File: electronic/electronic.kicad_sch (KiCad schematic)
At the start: 63 parts, among them J1 POWER SUPLY, J10 MOT_W_ENCODER03, J11 Conn_01x02, J12 Conn_01x02, J13 Conn_01x02, J14 DRVO01, J15 DRVO01, J16 Screw_Terminal_01x03, J17 Conn_01x04, J18 Conn_01x02, J19 Conn_01x02, J2 MOT_W_ENCODER01, J20 Conn_01x02, J21 DRVO01, J22 Screw_Terminal_01x03, J23 DRVO01, J24 Conn_01x04, J25 Conn_01x05, J26 Conn_01x04, J27 Conn_01x04, J28 Conn_01x05, J3 M01, J4 ENC01, J5 M02, J6 ENC02, J7 MOT_W_ENCODER02, J8 M03, J9 ENC03, U1 ESP32-S3-DevKitC, U2 L298N, U3 LM78M05_TO252, U4 L298N, U5 LM78M05_TO252

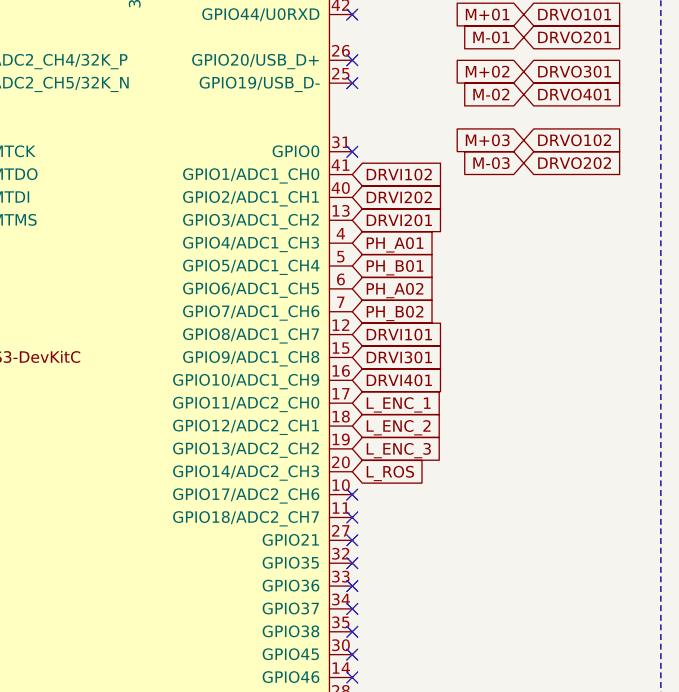
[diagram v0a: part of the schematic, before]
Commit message: chore: PCB updated
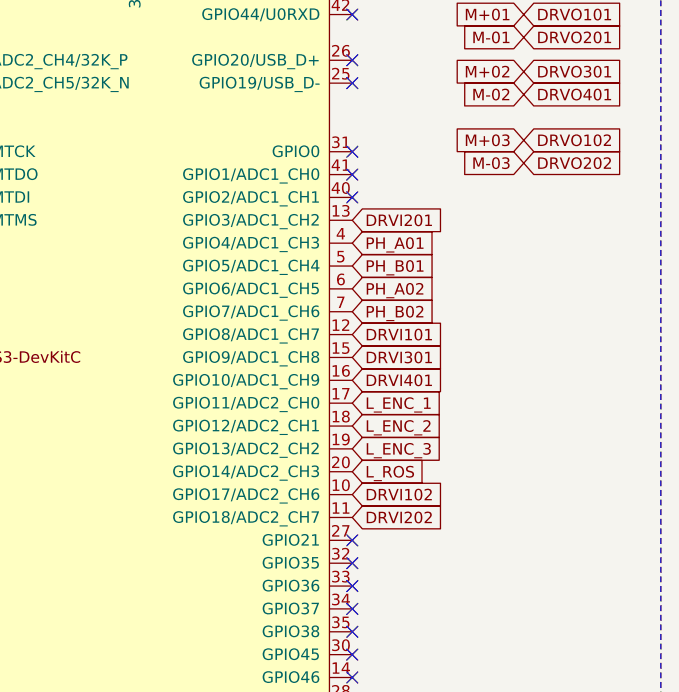
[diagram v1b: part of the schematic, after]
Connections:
- net DRVI102: now also U1.10 (GPIO17/ADC2_CH6); no longer U1.41 (GPIO1/ADC1_CH0)
- net DRVI202: now also U1.11 (GPIO18/ADC2_CH7); no longer U1.40 (GPIO2/ADC1_CH1)
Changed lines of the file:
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@@
 	)
 	(no_connect
+		(at 240.03 88.9)
+	)
+	(no_connect
 		(at 189.23 86.36)
 	)
@@
 	)
 	(no_connect
-		(at 240.03 121.92)
+		(at 240.03 142.24)
 	)
 	(no_connect
-		(at 240.03 142.24)
+		(at 240.03 86.36)
 	)
 	(no_connect
@@
 	)
 	(no_connect
-		(at 240.03 124.46)
-	)
-	(no_connect
 		(at 240.03 66.04)
 	)
@@
 		)
 	)
-	(global_label "DRVI202"
-		(shape input)
-		(at 240.03 88.9 0)
-		(fields_autoplaced yes)
-		(effects
-			(font
-				(size 1.27 1.27)
-			)
-			(justify left)
-		)
-		(property "Intersheetrefs" "${INTERSHEET_REFS}"
-			(at 250.8771 88.9 0)
-			(effects
-				(font
-					(size 1.27 1.27)
-				)
-				(justify left)
-				(hide yes)
-			)
-		)
-	)
 	(global_label "DRVO302"
 		(shape input)
@@
 		)
 	)
+	(global_label "DRVI202"
+		(shape input)
+		(at 240.03 124.46 0)
+		(fields_autoplaced yes)
+		(effects
+			(font
+				(size 1.27 1.27)
+			)
+			(justify left)
+		)
+		(property "Intersheetrefs" "${INTERSHEET_REFS}"
+			(at 250.8771 124.46 0)
+			(effects
+				(font
+					(size 1.27 1.27)
+				)
+				(justify left)
+				(hide yes)
+			)
+		)
+	)
 	(global_label "PH_A01"
 		(shape input)
@@
 		)
 	)
-	(global_label "DRVI102"
-		(shape input)
-		(at 240.03 86.36 0)
-		(fields_autoplaced yes)
-		(effects
-			(font
-				(size 1.27 1.27)
-			)
-			(justify left)
-		)
-		(property "Intersheetrefs" "${INTERSHEET_REFS}"
-			(at 250.8771 86.36 0)
-			(effects
-				(font
-					(size 1.27 1.27)
-				)
-				(justify left)
-				(hide yes)
-			)
-		)
-	)
 	(global_label "DRVI101"
 		(shape input)
@@
 				(hide yes)
 			)
+		)
+	)
+	(global_label "DRVI102"
+		(shape input)
+		(at 240.03 121.92 0)
+		(fields_autoplaced yes)
+		(effects
+			(font
+				(size 1.27 1.27)
+			)
+			(justify left)
+		)
+		(property "Intersheetrefs" "${INTERSHEET_REFS}"
+			(at 250.8771 121.92 0)
+			(effects
+				(font
+					(size 1.27 1.27)
+				)
+				(justify left)
+				(hide yes)
+			)
